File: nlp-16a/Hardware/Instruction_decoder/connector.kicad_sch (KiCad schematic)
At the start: 35 parts, among them J1 Conn_02x10_Odd_Even, J2 Conn_02x10_Odd_Even, J3 Screw_Terminal_01x02, J4 Conn_02x10_Counter_Clockwise, J5 Conn_02x10_Counter_Clockwise, U85 CD74HC00

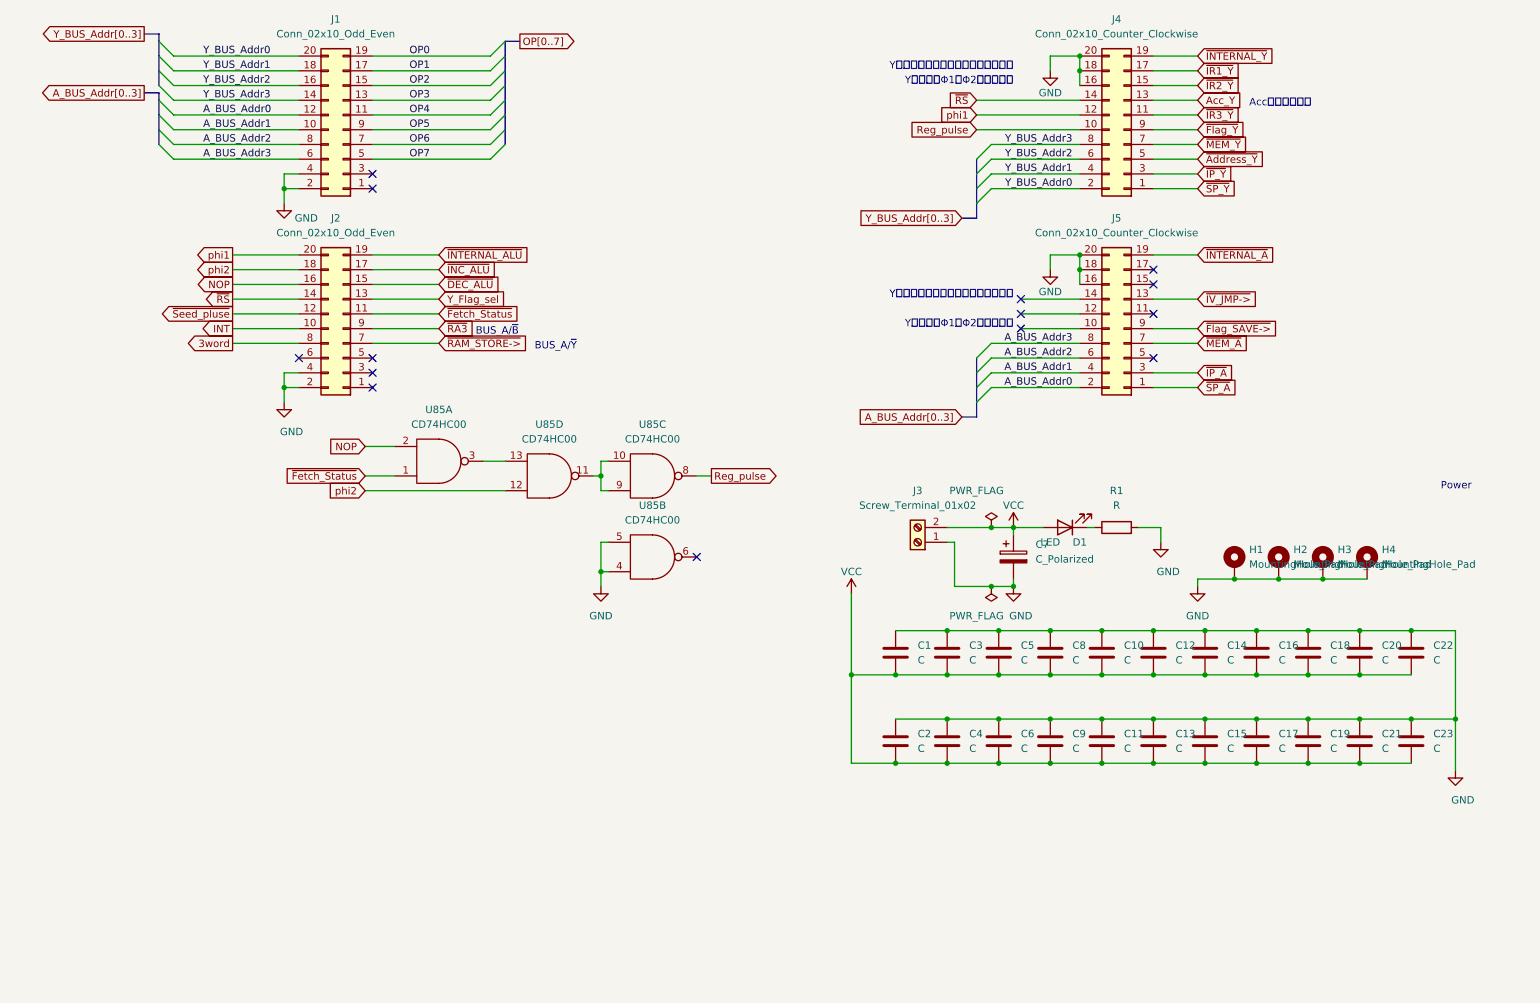
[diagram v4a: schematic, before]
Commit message: 命令デコーダ完了！！
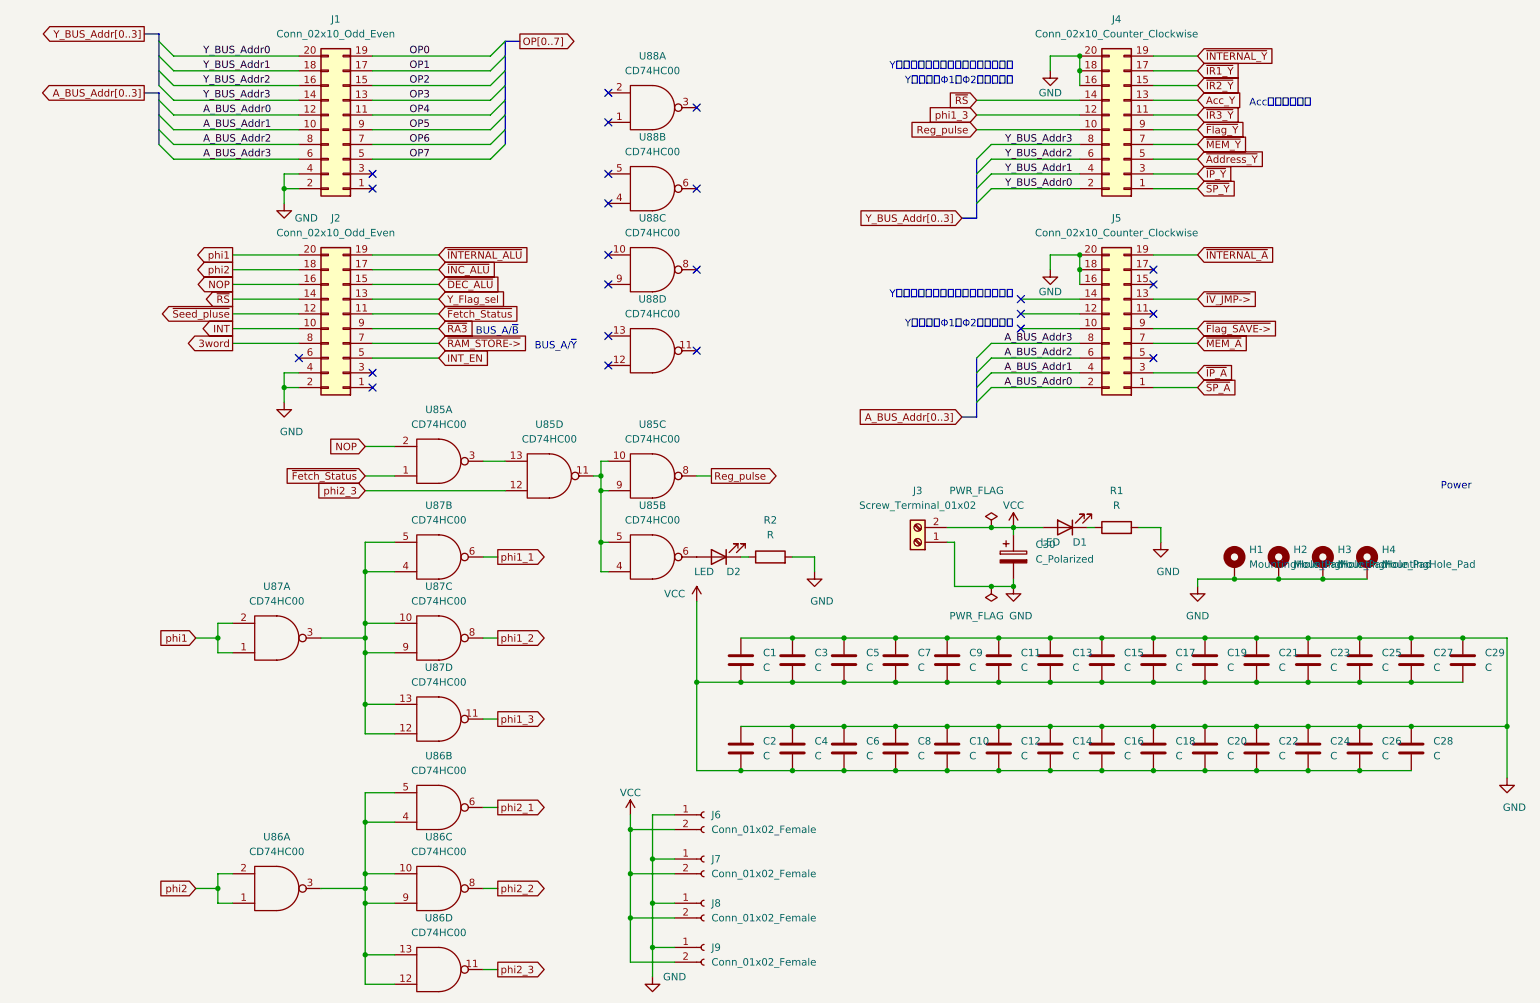
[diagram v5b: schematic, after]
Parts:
- added C23, C24, C25, C26, C27, C28, C29: C, Capacitor_THT:C_Disc_D7.0mm_W2.5mm_P5.00mm, symbol Device:C
- added D2: LED, LED_THT:LED_D3.0mm, symbol Device:LED
- added J6, J7, J8, J9: Conn_01x02_Female, Connector_PinSocket_2.54mm:PinSocket_1x02_P2.54mm_Vertical, symbol Connector:Conn_01x02_Female
- added R2: R, Resistor_SMD:R_0603_1608Metric_Pad0.98x0.95mm_HandSolder, symbol Device:R
- added U86, U87, U88: CD74HC00, Package_DIP:DIP-14_W7.62mm, symbol CD74HCXX:CD74HC00
- C1, C10, C11, C12, C13, C14, C15, C16, C17, C18, C19, C2, C20, C21, C22, C3, C4, C5, C6, C8, C9: footprint Capacitor_THT:C_Disc_D7.5mm_W2.5mm_P5.00mm -> Capacitor_THT:C_Disc_D7.0mm_W2.5mm_P5.00mm
- C7: renamed from C23; footprint Capacitor_THT:C_Disc_D7.5mm_W2.5mm_P5.00mm -> Capacitor_THT:C_Disc_D7.0mm_W2.5mm_P5.00mm
- renumbered C7 to C30
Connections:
- net GND: now also C23.1, C24.1, C25.1, C26.1, C27.1, C28.1, C29.1, J6.1 (Pin_1), J7.1 (Pin_1), J8.1 (Pin_1), J9.1 (Pin_1), R2.2, U86.7 (GND), U86.7 (GND), U86.7 (GND), U86.7 (GND), U87.7 (GND), U87.7 (GND), U87.7 (GND), U87.7 (GND), U88.7 (GND), U88.7 (GND), U88.7 (GND), U88.7 (GND); no longer U85.4, U85.5
- net VCC: now also C23.2, C24.2, C25.2, C26.2, C27.2, C28.2, C29.2, J6.2 (Pin_2), J7.2 (Pin_2), J8.2 (Pin_2), J9.2 (Pin_2), U86.14 (VCC), U86.14 (VCC), U86.14 (VCC), U86.14 (VCC), U87.14 (VCC), U87.14 (VCC), U87.14 (VCC), U87.14 (VCC), U88.14 (VCC), U88.14 (VCC), U88.14 (VCC), U88.14 (VCC)
- net phi1: now also U87.1, U87.2; no longer J4.12 (Pin_12)
- net phi2: now also U86.1, U86.2; no longer U85.12
- net INT_EN: now reaches J2.5 (Pin_5)
- net at U85.6: now also D2.2 (A)
- net at U85.10, U85.11, U85.9: now also U85.4, U85.5
- new net: U87.10, U87.12, U87.13, U87.3, U87.4, U87.5, U87.9
- new net: U86.10, U86.12, U86.13, U86.3, U86.4, U86.5, U86.9
- new net: D2.1 (K), R2.1
- new net phi1_1: U87.6
- new net phi1_2: U87.8
- new net phi1_3: J4.12 (Pin_12), U87.11
- new net phi2_1: U86.6
- new net phi2_2: U86.8
- new net phi2_3: U85.12, U86.11
- no-connect marks 14 -> 24
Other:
- moved on the sheet: C1, C10, C11, C12, C13, C14, C15, C16, C17, C18, C19, C2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
